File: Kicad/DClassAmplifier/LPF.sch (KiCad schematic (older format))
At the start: 9 parts

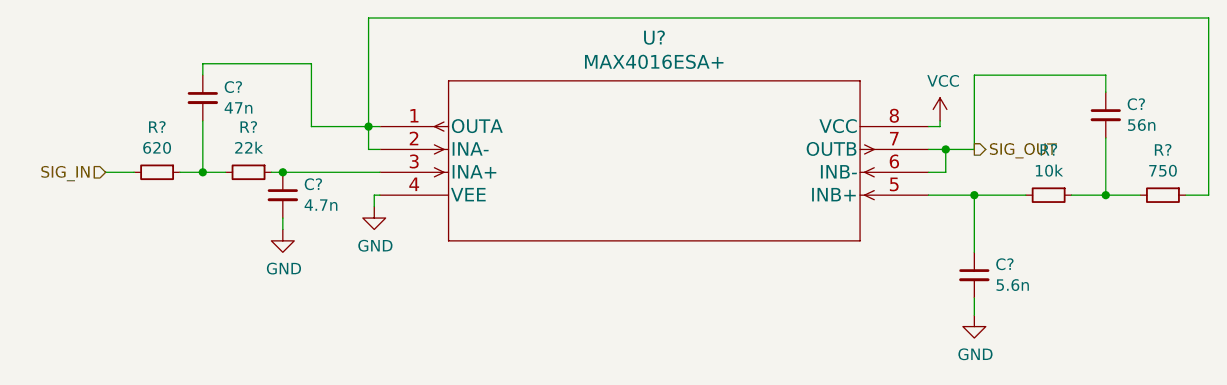
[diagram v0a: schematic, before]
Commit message: updates to schematic
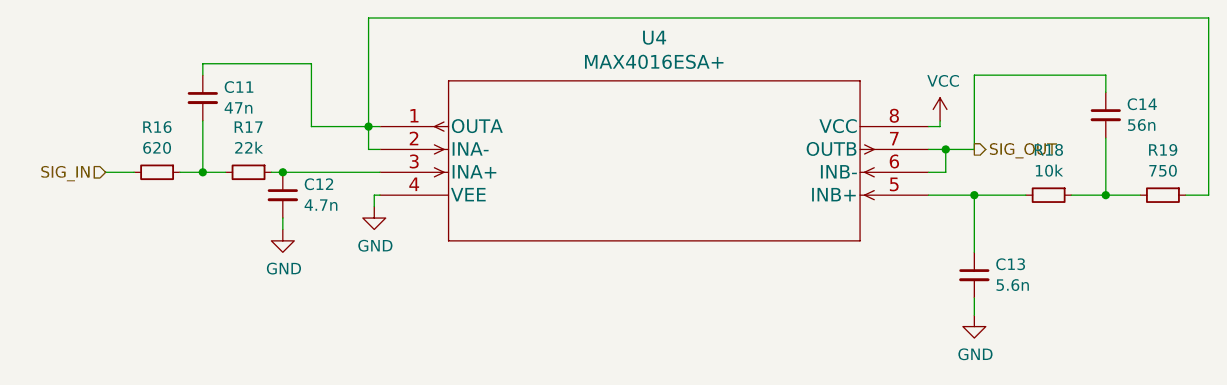
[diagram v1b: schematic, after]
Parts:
- gave numbers to parts that had none: 9
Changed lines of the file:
@@
 $EndDescr
 $Comp
-L MAX4016ESA:MAX4016ESA+ U?
+L MAX4016ESA:MAX4016ESA+ U4
 U 1 1 61194DD9
 P 7475 3225
-F 0 "U?" H 8675 3612 60  0000 C CNN
+F 0 "U4" H 8675 3612 60  0000 C CNN
 F 1 "MAX4016ESA+" H 8675 3506 60  0000 C CNN
 F 2 "21-0041B_8_MXM" H 8675 3465 60  0001 C CNN
@@
 $EndComp
 $Comp
-L power:VCC #PWR?
+L power:VCC #PWR0141
 U 1 1 61197634
 P 9925 3200
-F 0 "#PWR?" H 9925 3050 50  0001 C CNN
+F 0 "#PWR0141" H 9925 3050 50  0001 C CNN
 F 1 "VCC" H 9940 3373 50  0000 C CNN
 F 2 "" H 9925 3200 50  0001 C CNN
@@
 	9925 3225 9875 3225
 $Comp
-L power:GND #PWR?
+L power:GND #PWR0142
 U 1 1 61197F03
 P 7450 3575
-F 0 "#PWR?" H 7450 3325 50  0001 C CNN
+F 0 "#PWR0142" H 7450 3325 50  0001 C CNN
 F 1 "GND" H 7455 3402 50  0000 C CNN
 F 2 "" H 7450 3575 50  0001 C CNN
@@
 	7450 3525 7475 3525
 $Comp
-L Device:R_Small R?
+L Device:R_Small R17
 U 1 1 6119FD9F
 P 6900 3425
-F 0 "R?" V 6704 3425 50  0000 C CNN
+F 0 "R17" V 6704 3425 50  0000 C CNN
 F 1 "22k" V 6795 3425 50  0000 C CNN
 F 2 "Resistor_SMD:R_0603_1608Metric_Pad0.98x0.95mm_HandSolder" H 6900 3425 50  0001 C CNN
@@
 $EndComp
 $Comp
-L Device:R_Small R?
+L Device:R_Small R16
 U 1 1 611A0CB6
 P 6500 3425
-F 0 "R?" V 6304 3425 50  0000 C CNN
+F 0 "R16" V 6304 3425 50  0000 C CNN
 F 1 "620" V 6395 3425 50  0000 C CNN
 F 2 "Resistor_SMD:R_0603_1608Metric_Pad0.98x0.95mm_HandSolder" H 6500 3425 50  0001 C CNN
@@
 $EndComp
 $Comp
-L Device:C_Small C?
+L Device:C_Small C12
 U 1 1 611A751B
 P 7050 3525
-F 0 "C?" H 7142 3571 50  0000 L CNN
+F 0 "C12" H 7142 3571 50  0000 L CNN
 F 1 "4.7n" H 7142 3480 50  0000 L CNN
 F 2 "Capacitor_SMD:C_0603_1608Metric_Pad1.08x0.95mm_HandSolder" H 7050 3525 50  0001 C CNN
@@
 $EndComp
 $Comp
-L Device:C_Small C?
+L Device:C_Small C11
 U 1 1 611A7CBC
 P 6700 3100
-F 0 "C?" H 6792 3146 50  0000 L CNN
+F 0 "C11" H 6792 3146 50  0000 L CNN
 F 1 "47n" H 6792 3055 50  0000 L CNN
 F 2 "Capacitor_SMD:C_0603_1608Metric_Pad1.08x0.95mm_HandSolder" H 6700 3100 50  0001 C CNN
@@
 	7050 3625 7050 3675
 $Comp
-L power:GND #PWR?
+L power:GND #PWR0143
 U 1 1 611AAC29
 P 7050 3675
-F 0 "#PWR?" H 7050 3425 50  0001 C CNN
+F 0 "#PWR0143" H 7050 3425 50  0001 C CNN
 F 1 "GND" H 7055 3502 50  0000 C CNN
 F 2 "" H 7050 3675 50  0001 C CNN
@@
 	7425 3225 7175 3225
 $Comp
-L Device:C_Small C?
+L Device:C_Small C13
 U 1 1 611BBE57
 P 10075 3875
-F 0 "C?" H 10167 3921 50  0000 L CNN
+F 0 "C13" H 10167 3921 50  0000 L CNN
 F 1 "5.6n" H 10167 3830 50  0000 L CNN
 F 2 "Capacitor_SMD:C_0603_1608Metric_Pad1.08x0.95mm_HandSolder" H 10075 3875 50  0001 C CNN
@@
 $EndComp
 $Comp
-L Device:R_Small R?
+L Device:R_Small R18
 U 1 1 611BC850
 P 10400 3525
-F 0 "R?" V 10204 3525 50  0000 C CNN
+F 0 "R18" V 10204 3525 50  0000 C CNN
 F 1 "10k" V 10295 3525 50  0000 C CNN
 F 2 "Resistor_SMD:R_0603_1608Metric_Pad0.98x0.95mm_HandSolder" H 10400 3525 50  0001 C CNN
@@
 $EndComp
 $Comp
-L Device:R_Small R?
+L Device:R_Small R19
 U 1 1 611BD0E0
 P 10900 3525
-F 0 "R?" V 10704 3525 50  0000 C CNN
+F 0 "R19" V 10704 3525 50  0000 C CNN
 F 1 "750" V 10795 3525 50  0000 C CNN
 F 2 "Resistor_SMD:R_0603_1608Metric_Pad0.98x0.95mm_HandSolder" H 10900 3525 50  0001 C CNN
@@
 	11100 3525 11000 3525
 $Comp
-L Device:C_Small C?
+L Device:C_Small C14
 U 1 1 611C0153
 P 10650 3175
-F 0 "C?" H 10742 3221 50  0000 L CNN
+F 0 "C14" H 10742 3221 50  0000 L CNN
 F 1 "56n" H 10742 3130 50  0000 L CNN
 F 2 "Capacitor_SMD:C_0603_1608Metric_Pad1.08x0.95mm_HandSolder" H 10650 3175 50  0001 C CNN
@@
 	10650 3525 10800 3525
 $Comp
-L power:GND #PWR?
+L power:GND #PWR0144
 U 1 1 611C31DE
 P 10075 4050
-F 0 "#PWR?" H 10075 3800 50  0001 C CNN
+F 0 "#PWR0144" H 10075 3800 50  0001 C CNN
 F 1 "GND" H 10080 3877 50  0000 C CNN
 F 2 "" H 10075 4050 50  0001 C CNN
